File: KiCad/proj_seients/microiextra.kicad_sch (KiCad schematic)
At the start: 63 parts, among them J10 Screw_Terminal_01x05, J11 FCarrera, J12 FCarrera, J13 FCarrera, J14 FCarrera, J17 FCarrera, J2 5f0857756ylz, J3 DE9_Pins, J8 DE9_Socket, J9 FCarrera, SW1 SW_Push, SW2 SW_Push, SW3 SW_Push, SW4 SW_Push, SW5 SW_Push, SW6 SW_Push, SW7 SW_Push, U1 PIC24HJ128GP502, U10 MAX3232, U11 PCF8574AP, U4 MCP2562-E-SN, U9 24LC256, Y1 8MHz

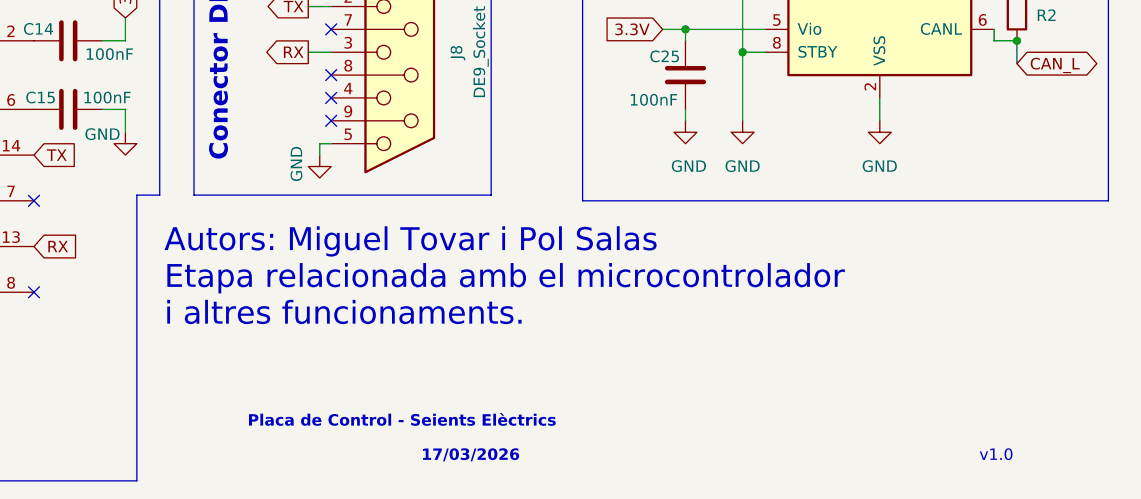
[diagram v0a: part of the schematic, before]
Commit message: Versió 1.0 Layout
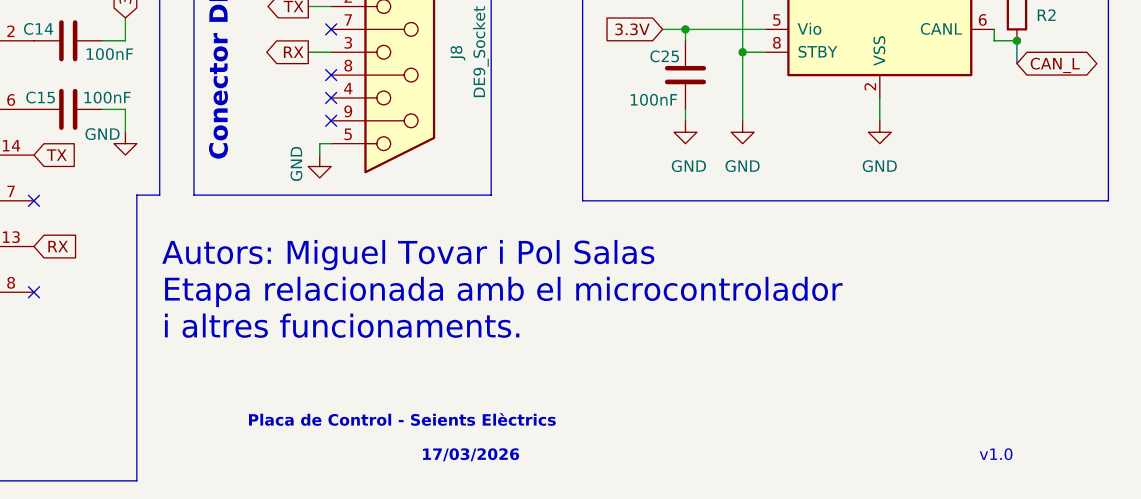
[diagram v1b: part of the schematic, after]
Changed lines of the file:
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@@
 	(text "Autors: Miguel Tovar i Pol Salas\nEtapa relacionada amb el microcontrolador \ni altres funcionaments.\n"
 		(exclude_from_sim no)
-		(at 178.308 173.736 0)
+		(at 178.054 175.26 0)
 		(effects
 			(font

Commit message: Exclusió de dos errors justificats
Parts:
- J3: footprint Connector_Dsub:DSUB-9_Pins_Vertical_P2.77x2.84mm -> Connector_Dsub:DSUB-9_Pins_Horizontal_P2.77x2.84mm_EdgePinOffset9.40mm
- J8: footprint Connector_Dsub:DSUB-9_Socket_Vertical_P2.77x2.84mm -> Connector_Dsub:DSUB-9_Socket_Horizontal_P2.77x2.84mm_EdgePinOffset9.40mm
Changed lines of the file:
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@@
 			)
 		)
-		(property "Footprint" "Connector_Dsub:DSUB-9_Pins_Vertical_P2.77x2.84mm"
+		(property "Footprint" "Connector_Dsub:DSUB-9_Pins_Horizontal_P2.77x2.84mm_EdgePinOffset9.40mm"
 			(at 270.51 99.06 0)
 			(effects
@@
 			)
 		)
-		(property "Footprint" "Connector_Dsub:DSUB-9_Socket_Vertical_P2.77x2.84mm"
+		(property "Footprint" "Connector_Dsub:DSUB-9_Socket_Horizontal_P2.77x2.84mm_EdgePinOffset9.40mm"
 			(at 204.47 148.59 0)
 			(effects

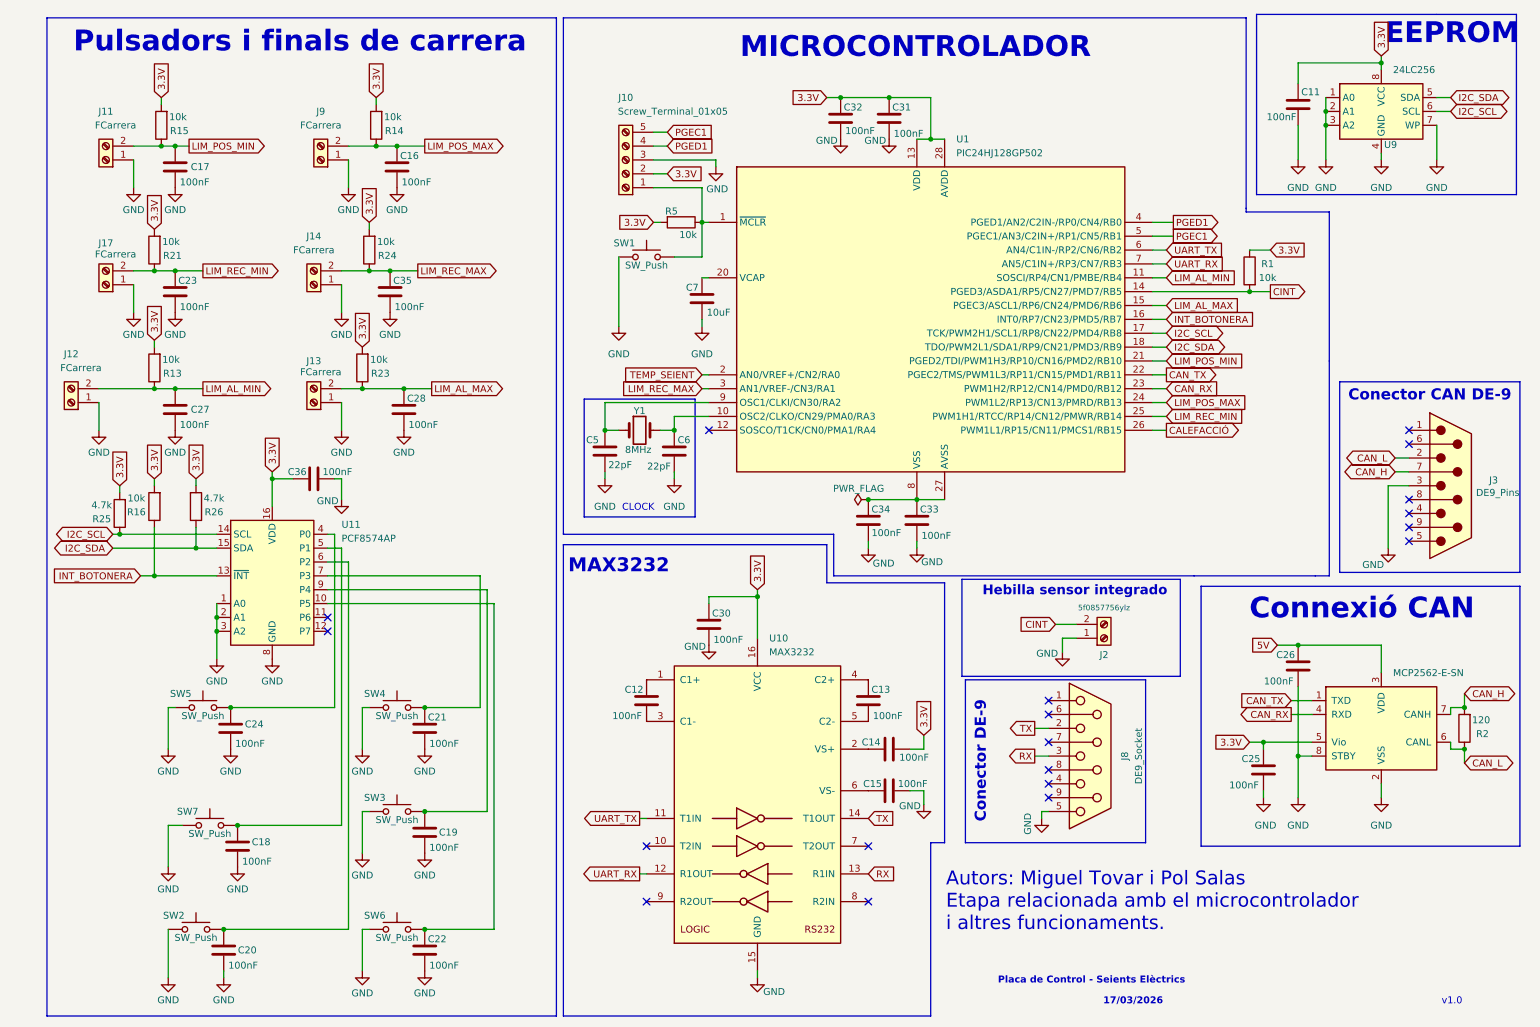
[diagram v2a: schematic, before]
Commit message: V3.2
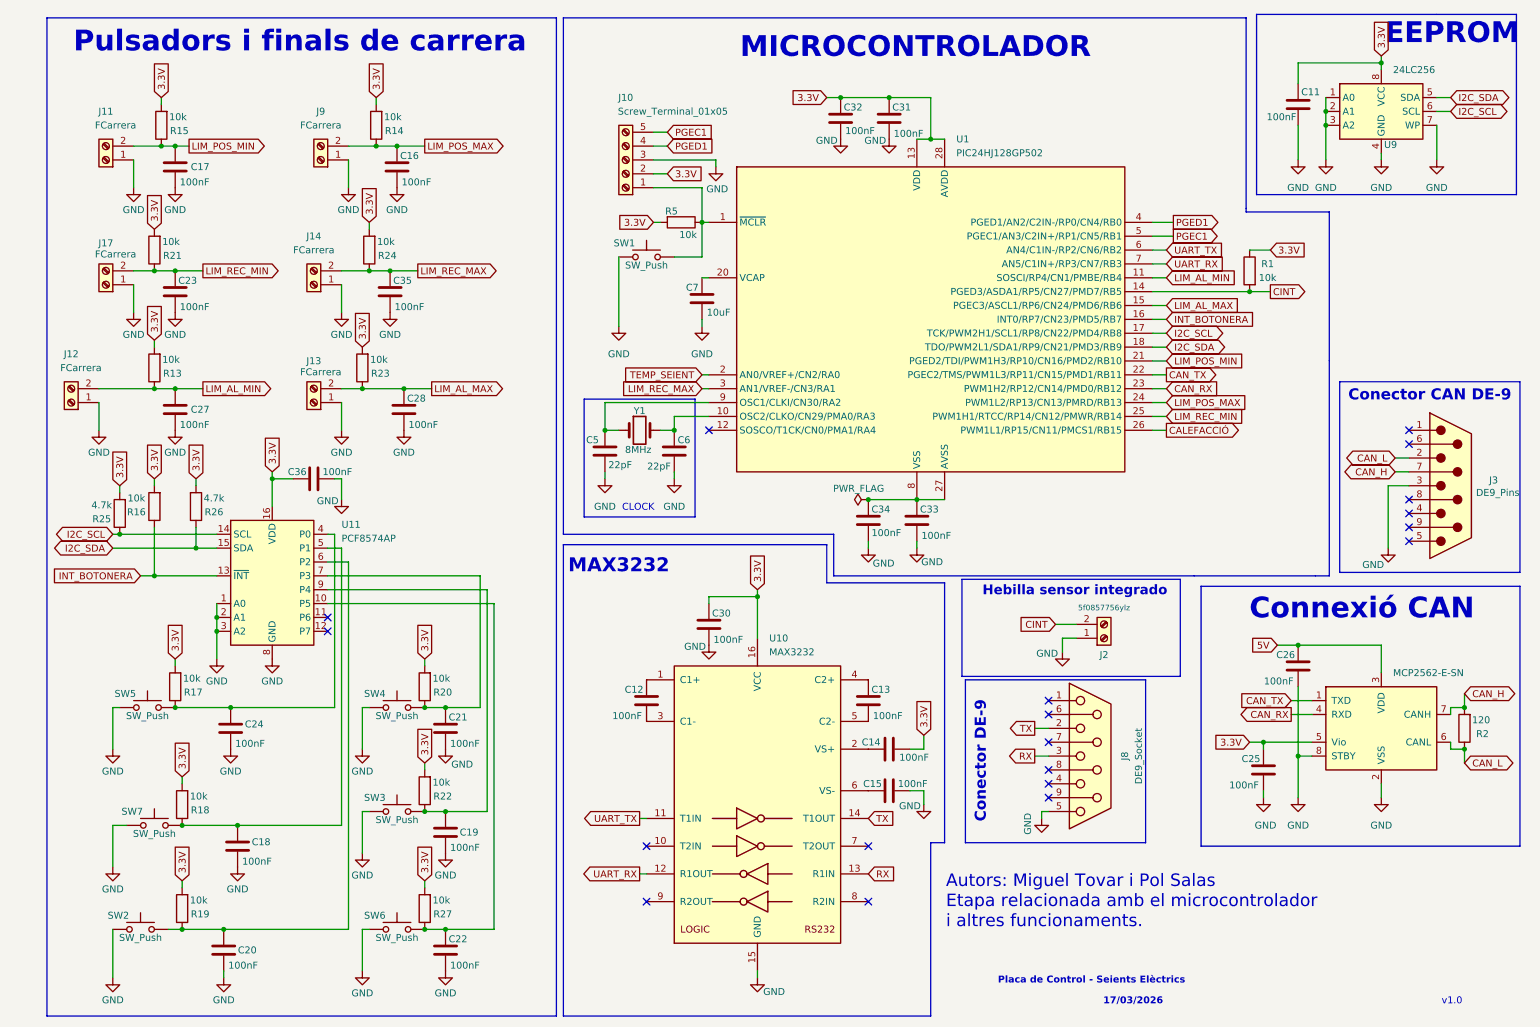
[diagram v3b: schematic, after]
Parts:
- added R17, R18, R19, R20, R22, R27: 10k, Resistor_SMD:R_0805_2012Metric, symbol Device:R
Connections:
- net 3.3V: now also R17.2, R18.2, R19.2, R20.2, R22.2, R27.2
- net at C18.2, SW7.2, U11.5 (P1): now also R18.1
- net at C21.2, SW4.2, U11.7 (P3): now also R20.1
- net at C24.2, SW5.2, U11.4 (P0): now also R17.1
- net at C19.2, SW3.2, U11.9 (P4): now also R22.1
- net at C22.2, SW6.2, U11.10 (P5): now also R27.1
- net at C20.2, SW2.2, U11.6 (P2): now also R19.1
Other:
- moved on the sheet: C19, C21, C22, SW2, SW5, SW7

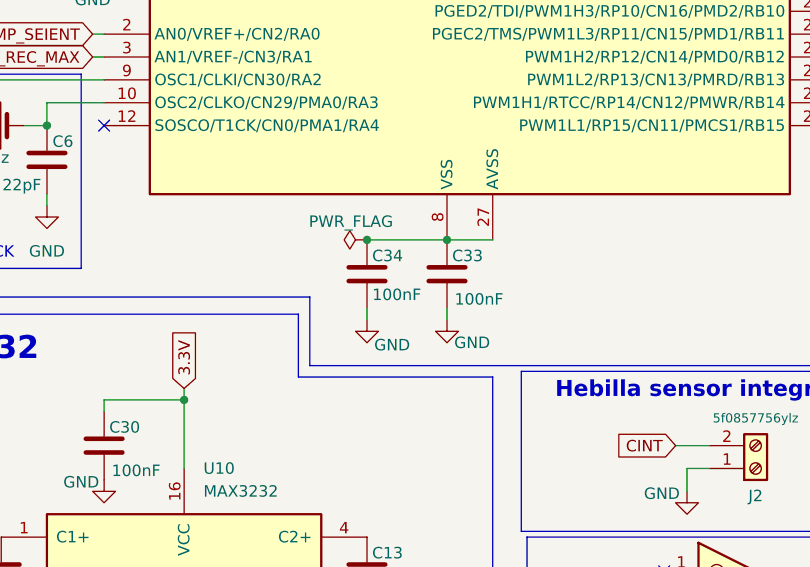
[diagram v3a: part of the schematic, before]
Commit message: V3.7
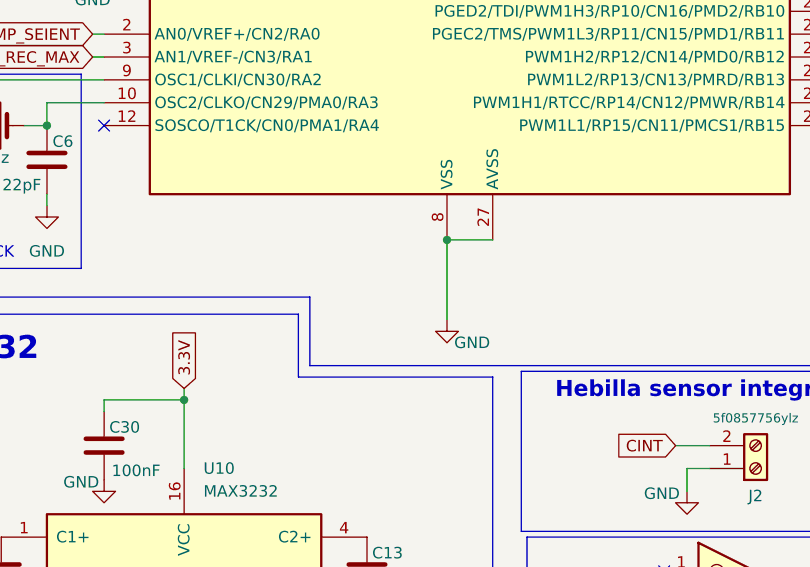
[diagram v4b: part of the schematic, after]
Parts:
- removed C33, C34: 100nF, Capacitor_SMD:C_0805_2012Metric, symbol Device:C
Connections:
- net GND: now also U1.19 (VSS), U1.27 (AVSS), U1.8 (VSS)

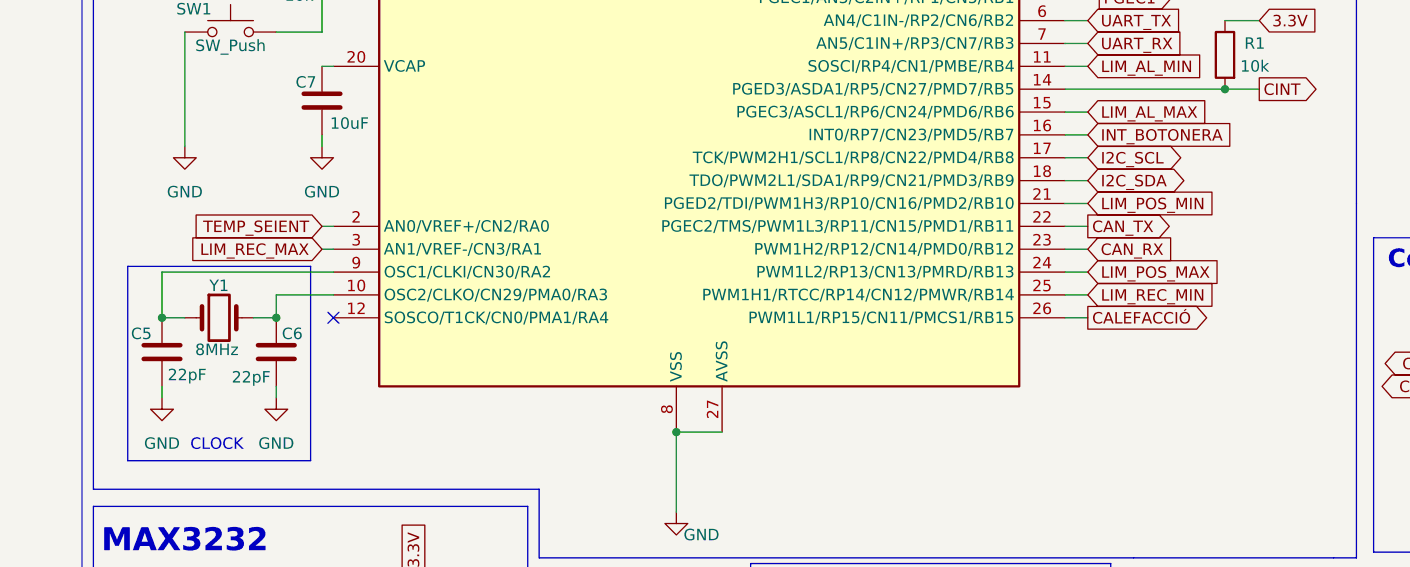
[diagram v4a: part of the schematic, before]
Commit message: V3.8
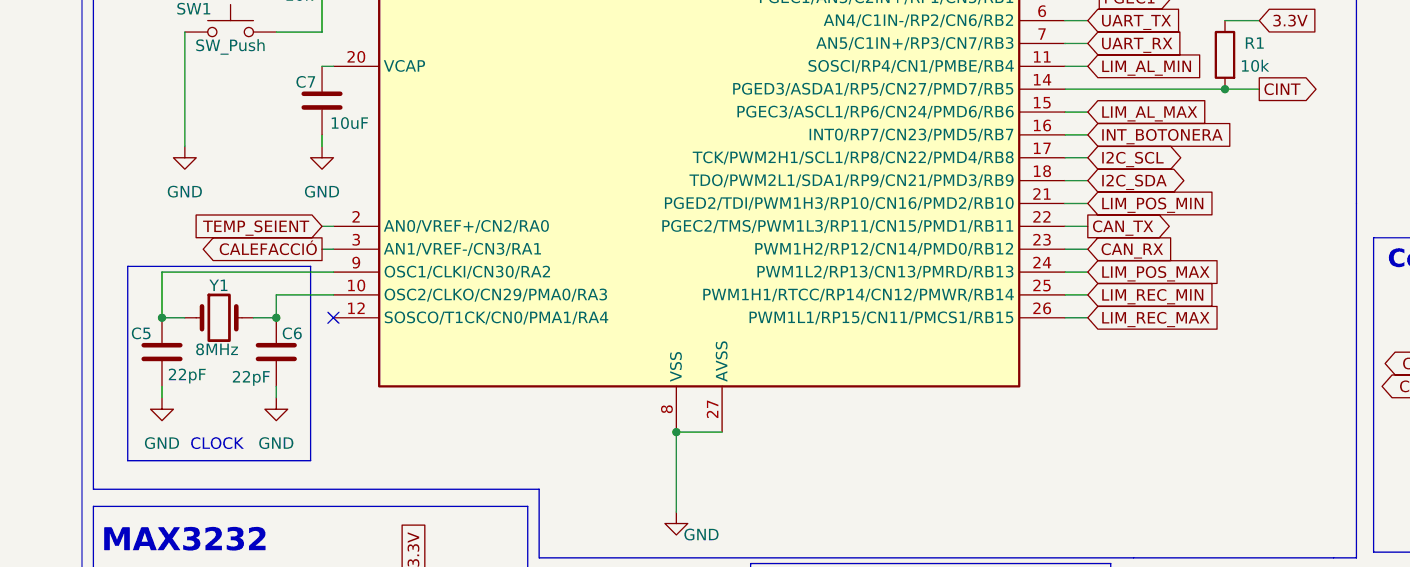
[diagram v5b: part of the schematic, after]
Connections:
- net CALEFACCIÓ: now also U1.3 (AN1/VREF-/CN3/RA1); no longer U1.26 (PWM1L1/RP15/CN11/PMCS1/RB15)
- net LIM_REC_MAX: now also U1.26 (PWM1L1/RP15/CN11/PMCS1/RB15); no longer U1.3 (AN1/VREF-/CN3/RA1)
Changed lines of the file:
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@@
 	(global_label "LIM_REC_MAX"
 		(shape input)
-		(at 133.35 81.28 180)
-		(fields_autoplaced yes)
-		(effects
-			(font
-				(size 1.27 1.27)
-			)
-			(justify right)
-		)
-		(property "Intersheetrefs" "${INTERSHEET_REFS}"
-			(at 117.9068 81.28 0)
-			(effects
-				(font
-					(size 1.27 1.27)
-				)
-				(justify right)
+		(at 218.44 88.9 0)
+		(fields_autoplaced yes)
+		(effects
+			(font
+				(size 1.27 1.27)
+			)
+			(justify left)
+		)
+		(property "Intersheetrefs" "${INTERSHEET_REFS}"
+			(at 233.8832 88.9 0)
+			(effects
+				(font
+					(size 1.27 1.27)
+				)
+				(justify left)
 				(hide yes)
 			)
@@
 	(global_label "CALEFACCIÓ"
 		(shape output)
-		(at 218.44 88.9 0)
-		(fields_autoplaced yes)
-		(effects
-			(font
-				(size 1.27 1.27)
-			)
-			(justify left)
-		)
-		(property "Intersheetrefs" "${INTERSHEET_REFS}"
-			(at 232.6134 88.9 0)
-			(effects
-				(font
-					(size 1.27 1.27)
-				)
-				(justify left)
-				(hide yes)
-			)
+		(at 133.35 81.28 180)
+		(fields_autoplaced yes)
+		(effects
+			(font
+				(size 1.27 1.27)
+			)
+			(justify right)
+		)
+		(property "Intersheetrefs" "${INTERSHEET_REFS}"
+			(at 119.1766 81.28 0)
+			(effects
+				(font
+					(size 1.27 1.27)
+				)
+				(justify right)
+				(hide yes)
+			)
